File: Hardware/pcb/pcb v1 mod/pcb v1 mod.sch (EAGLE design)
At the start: 48 parts, among them K1 JS-M1-9V-4, K2 JS-M1-9V-4, Q1 32.768kHz 12.5pF, Q10 MOSFET-NCHANNELBSS138, Q3 MOSFET-NCHANNELBSS138, Q4 MOSFET-NCHANNELBSS138, Q5 MOSFET-NCHANNELBSS138, Q6 MOSFET-NCHANNELBSS138, Q7 MOSFET-NCHANNELBSS138, Q8 MOSFET-NCHANNELBSS138, Q9 MOSFET-NCHANNELBSS138, U1 ADP3338AKCZ-3.3RL7

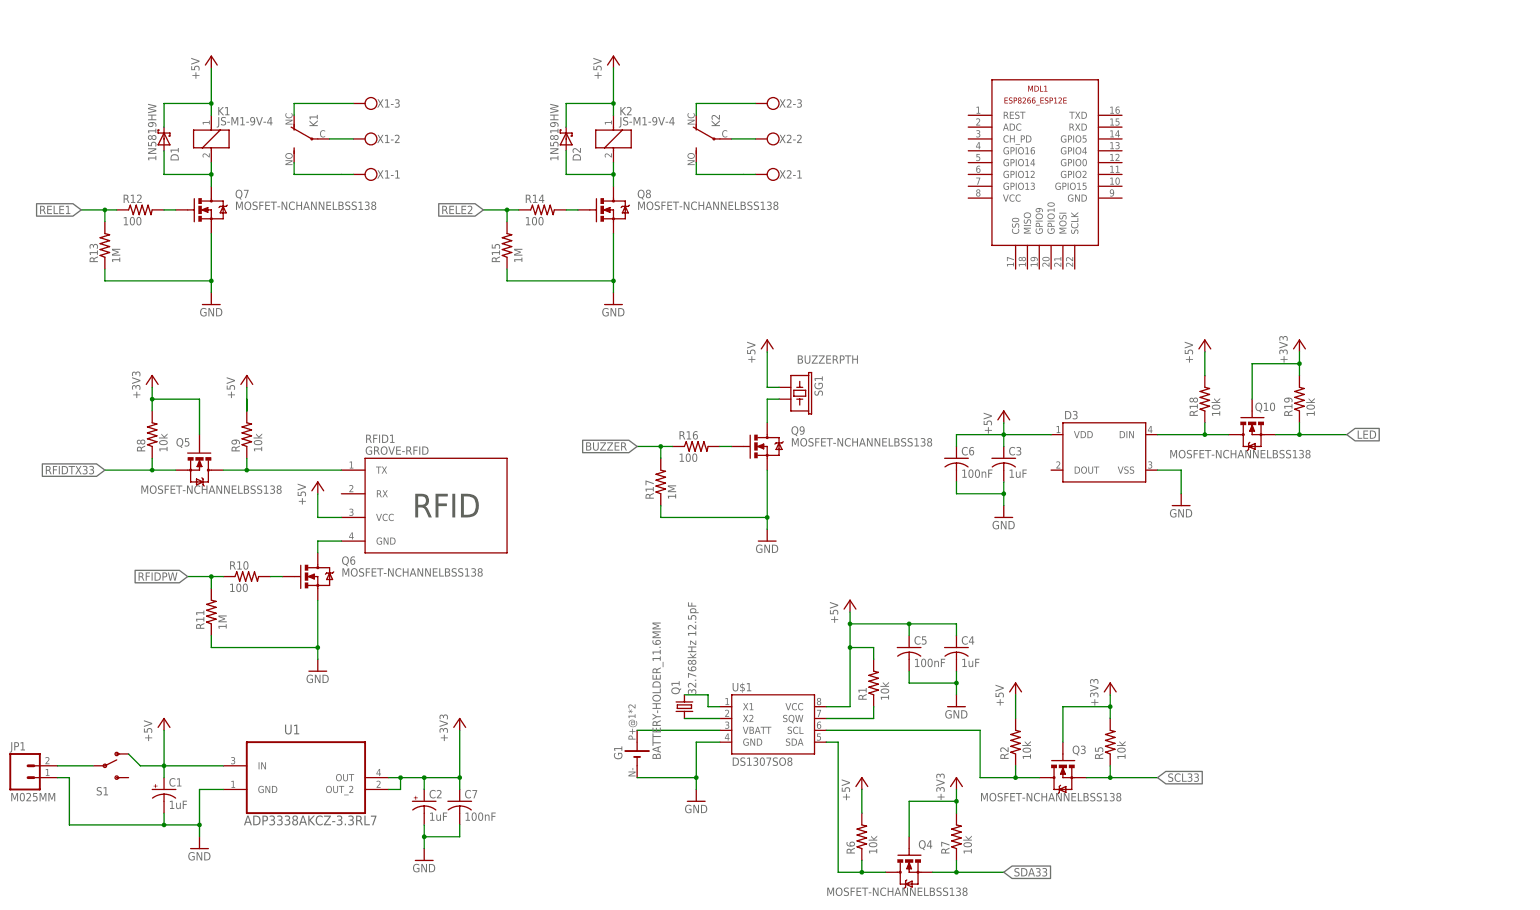
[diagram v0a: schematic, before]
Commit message: Ruteo completo
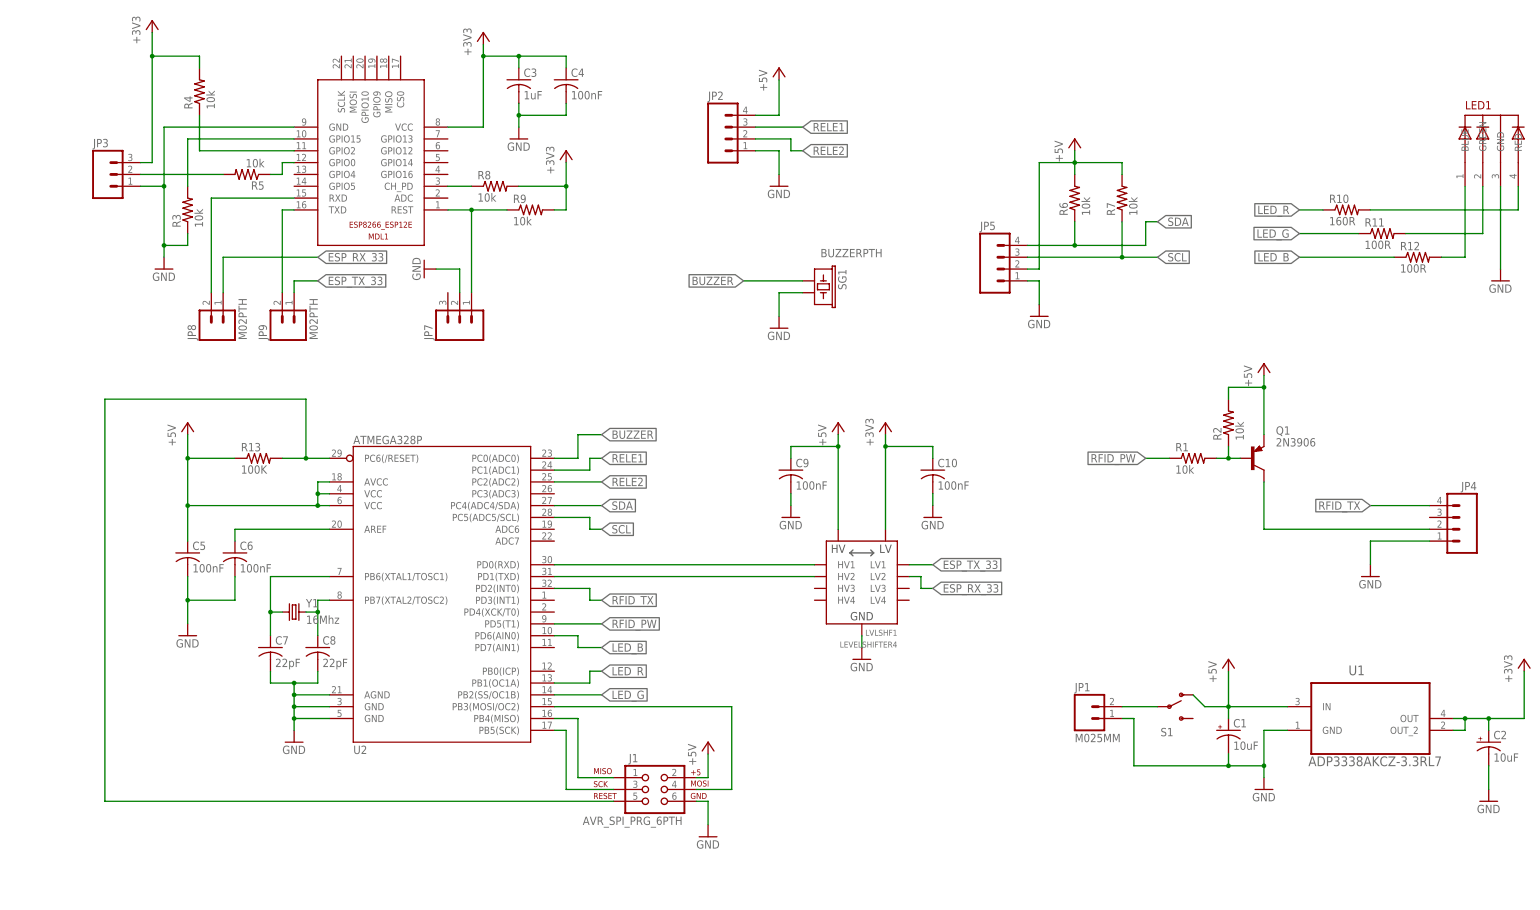
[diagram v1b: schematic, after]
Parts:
- removed D1, D2: 1N5819HW, diego:1N5819HW
- removed D3: (no value), SparkFun-LED:WS2812B
- removed G1: BATTERY-HOLDER_11.6MM, battery:BATTERY-HOLDER_11.6MM
- removed K1, K2: JS-M1-9V-4, relay:JS-M1-9V-4
- removed Q10, Q3, Q4, Q5, Q6, Q7, Q8, Q9: MOSFET-NCHANNELBSS138, SparkFun-DiscreteSemi:MOSFET-NCHANNELBSS138
- removed R14, R16: 100, rcl:R-US_R0805
- removed R15, R17: 1M, rcl:R-US_R0805
- removed R18, R19: 10k, rcl:R-US_R0805
- removed RFID1: GROVE-RFID, partes:GROVE-RFID
- removed U$1: DS1307SO8, SparkFun-FreqCtrl:DS1307SO8
- removed X1, X2: (no value), con-wago-500:W237-103
- added C10, C9: 100nF, rcl:C-USC0805
- added C8: 22pF, rcl:C-USC1206
- added J1: AVR_SPI_PRG_6PTH, SparkFun-Connectors:AVR_SPI_PRG_6PTH
- added JP2, JP4, JP5: (no value), SparkFun-Connectors:M041X04_NO_SILK
- added JP3, JP7: (no value), SparkFun-Connectors:M03PTH
- added JP8, JP9: M02PTH, SparkFun-Connectors:M02PTH
- added LED1: 5MMRGBLED, adafruit:5MMRGBLED
- added LVLSHF1: LEVELSHIFTER4, partes:LEVELSHIFTER4
- added R3, R4: 10k, rcl:R-US_R0805
- added U2: ATMEGA328P, SparkFun-DigitalIC:ATMEGA328_SMT
- added Y1: 16Mhz, SparkFun-FreqCtrl:CRYSTALHC49US
- C1, C2: value 1uF -> 10uF; device rcl:CPOL-US150CLZ-1010 -> rcl:CPOL-USE2.5-6
- C3: device rcl:C-USC0805 -> rcl:C-USC1206
- C4: value 1uF -> 100nF
- C7: value 100nF -> 22pF; device rcl:C-USC0805 -> rcl:C-USC1206
- Q1: value 32.768kHz 12.5pF -> 2N3906; device crystal:CRYSTALTC26H -> transistor-pnp:2N3906
- R10: value 100 -> 160R; device rcl:R-US_R0805 -> rcl:R-US_R1206
- R11: value 1M -> 100R
- R12: value 100 -> 100R
- R13: value 1M -> 100K
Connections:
- removed net LED: Q10.S, R19.1
- removed net N$13: Q6.G, R10.2
- removed net N$24: Q9.D, SG1.2
- removed net N$26: D3.DIN, Q10.D, R18.1
- removed net RFIDPW: R10.1, R11.2
- removed net RFIDTX33: Q5.S, R8.1
- removed net SCL33: Q3.S, R5.1
- removed net SDA33: Q4.S, R7.1
- new net AT_RST: J1.5, R13.2, U2.PC6(/RESET)
- new net ESP_RX_33: JP8.1, LVLSHF1.LV2
- new net ESP_TX_33: JP9.1, LVLSHF1.LV1
- new net LED_B: R12.1, U2.PD6(AIN0)
- new net LED_G: R11.1, U2.PB2(SS/OC1B)
- new net LED_R: R10.1, U2.PB1(OC1A)
- new net N$10: LED1.RED, R10.2
- new net N$8: JP9.2, MDL1.TXD
- new net RFID_PW: R1.1, U2.PD5(T1)
- new net RFID_TX: JP4.4, U2.PD2(INT0)
- new net SCL: JP5.3, R7.1, U2.PC5(ADC5/SCL)
- new net SDA: JP5.4, R6.1, U2.PC4(ADC4/SDA)
- net +3V3: now also C10.1, C3.1, C4.1, JP3.3, LVLSHF1.LV, MDL1.VCC, R4.2, R9.2; no longer C7.1, Q10.G, Q3.G, Q4.G, Q5.G, R19.2, R5.2, R7.2
- net +5V: now also C9.1, J1.2, JP2.4, JP5.2, LVLSHF1.HV, Q1.E, R13.1, R7.2, U2.AVCC, U2.VCC@1, U2.VCC@2; no longer C3.1, C4.1, C6.1, D1.C, D2.C, D3.VDD, K11.1, K21.1, R1.2, R18.2, R9.2, RFID1.VCC, SG1.1, U$1.VCC
- net BUZZER: now also SG1.1, U2.PC0(ADC0); no longer R16.1, R17.2
- net GND: now also C10.2, C8.2, C9.2, J1.6, JP2.1, JP3.1, JP4.1, JP5.1, JP7.2, LED1.GND, LVLSHF1.GND, MDL1.GND, R3.1, SG1.2, U2.AGND, U2.GND@1, U2.GND@2; no longer D3.VSS, G1.-, Q6.S, Q7.S, Q8.S, Q9.S, R11.1, R13.1, R15.1, R17.1, U$1.GND
- net N$11: now also C7.1, U2.PB6(XTAL1/TOSC1), Y1.1; no longer Q5.D, R9.1, RFID1.TX
- net N$12: now also C8.1, U2.PB7(XTAL2/TOSC2), Y1.2; no longer D1.A, K11.2, Q7.D
- net N$14: now also C6.1, U2.AREF; no longer Q7.G, R12.2
- net N$15: now also LED1.GREEN, R11.2; no longer K12.O, X1-3.KL
- net N$16: now also LED1.BLUE, R12.2; no longer K12.P, X1-2.KL
- net N$17: now also J1.3, U2.PB5(SCK); no longer K12.S, X1-1.KL
- net N$18: now also J1.1, U2.PB4(MISO); no longer D2.A, K21.2, Q8.D
- net N$19: now also J1.4, U2.PB3(MOSI/OC2); no longer Q8.G, R14.2
- net N$2: now also MDL1.CH_PD, R8.1; no longer Q1.2, U$1.X1
- net N$20: now also JP3.2, R5.2; no longer K22.O, X2-3.KL
- net N$21: now also LVLSHF1.HV1, U2.PD0(RXD); no longer K22.P, X2-2.KL
- net N$22: now also LVLSHF1.HV2, U2.PD1(TXD); no longer K22.S, X2-1.KL
- net N$23: now also JP4.2, Q1.C; no longer Q9.G, R16.2
- net N$3: now also MDL1.GPIO2, R4.1; no longer Q1.1, U$1.X2
- net N$4: now also MDL1.GPIO0, R5.1; no longer G1.+, U$1.VBATT
- net N$5: now also MDL1.GPIO15, R3.2; no longer Q3.D, R2.1, U$1.SCL
- net N$6: now also JP8.2, MDL1.RXD; no longer R1.1, U$1.SQW
- net N$7: now also Q1.B, R1.2, R2.1; no longer Q6.D, RFID1.GND
- net N$9: now also JP7.1, MDL1.REST, R9.1; no longer Q4.D, R6.1, U$1.SDA
- net RELE1: now also JP2.3, U2.PC1(ADC1); no longer R12.1, R13.2
- net RELE2: now also JP2.2, U2.PC2(ADC2); no longer R14.1, R15.2
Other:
- moved on the sheet: C1, C2, C3, C4, C5, C6, C7, JP1, MDL1, R1, R10, R11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
